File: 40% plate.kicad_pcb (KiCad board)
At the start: 2 copper layers, 230.2 x 98.4 mm, 47 parts, among them j1 MX-NoLED

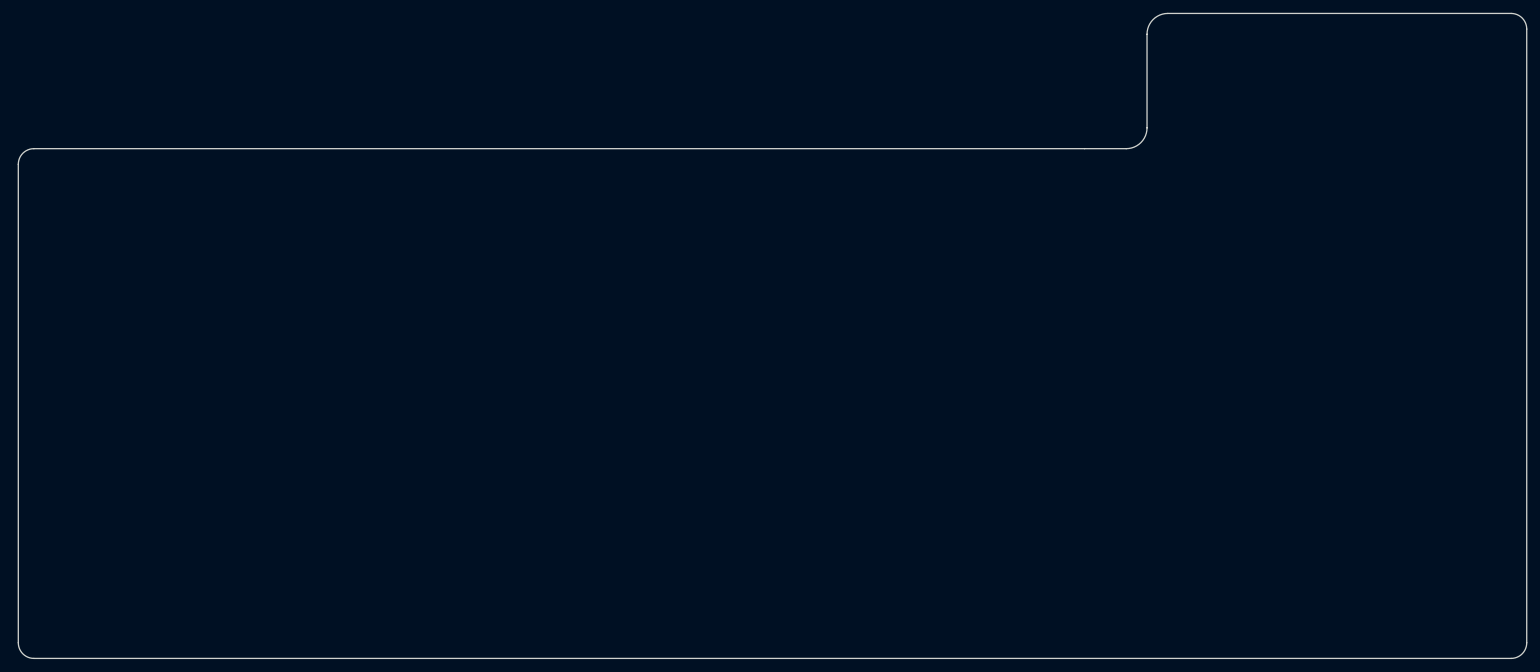
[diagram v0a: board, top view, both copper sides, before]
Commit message: finalized some things, slight edits to prep for production
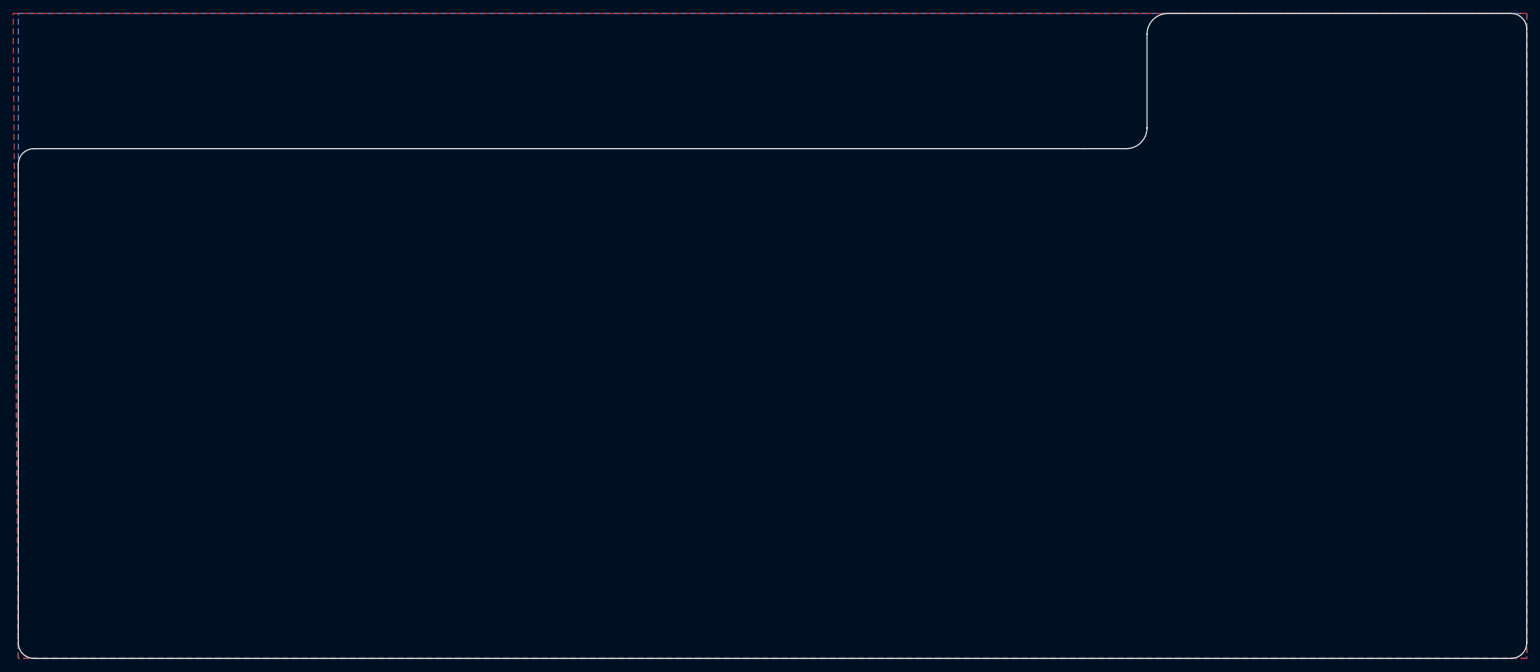
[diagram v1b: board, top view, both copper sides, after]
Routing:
- added copper zone on B.Cu, net (none)
- added copper zone on F.Cu, net (none)
